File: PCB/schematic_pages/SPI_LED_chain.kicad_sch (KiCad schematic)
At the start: 55 parts

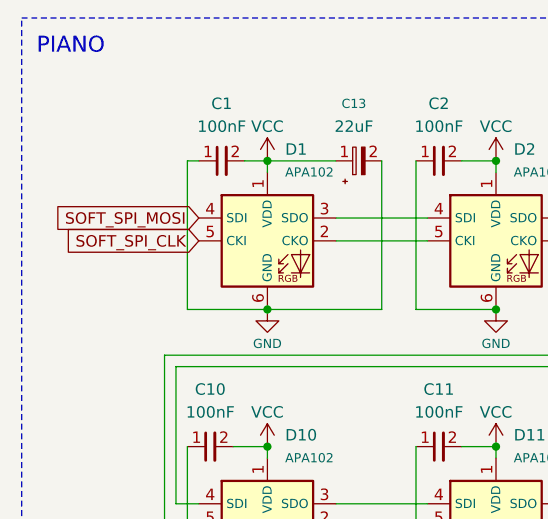
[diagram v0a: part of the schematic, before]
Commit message: repo rearrange
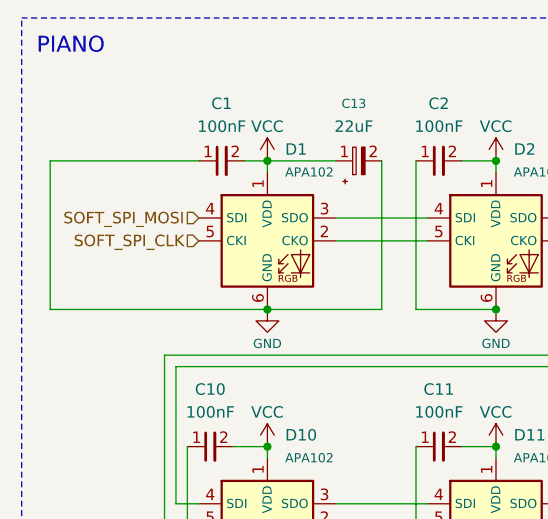
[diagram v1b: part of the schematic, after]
